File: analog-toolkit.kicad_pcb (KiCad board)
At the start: 2 copper layers, 50 x 36 mm, 54 parts, among them J1 USB_C, J2 IO, J3 UART, J4 I2C, J5 VBUS, J6 3.3V, J7 OPAMP, J8 ADC, P1 TC2030, SW1 DFU, U1 AP2204R-3.3, U2 otter_USBLC6-4, U3 STM32G431KBT6

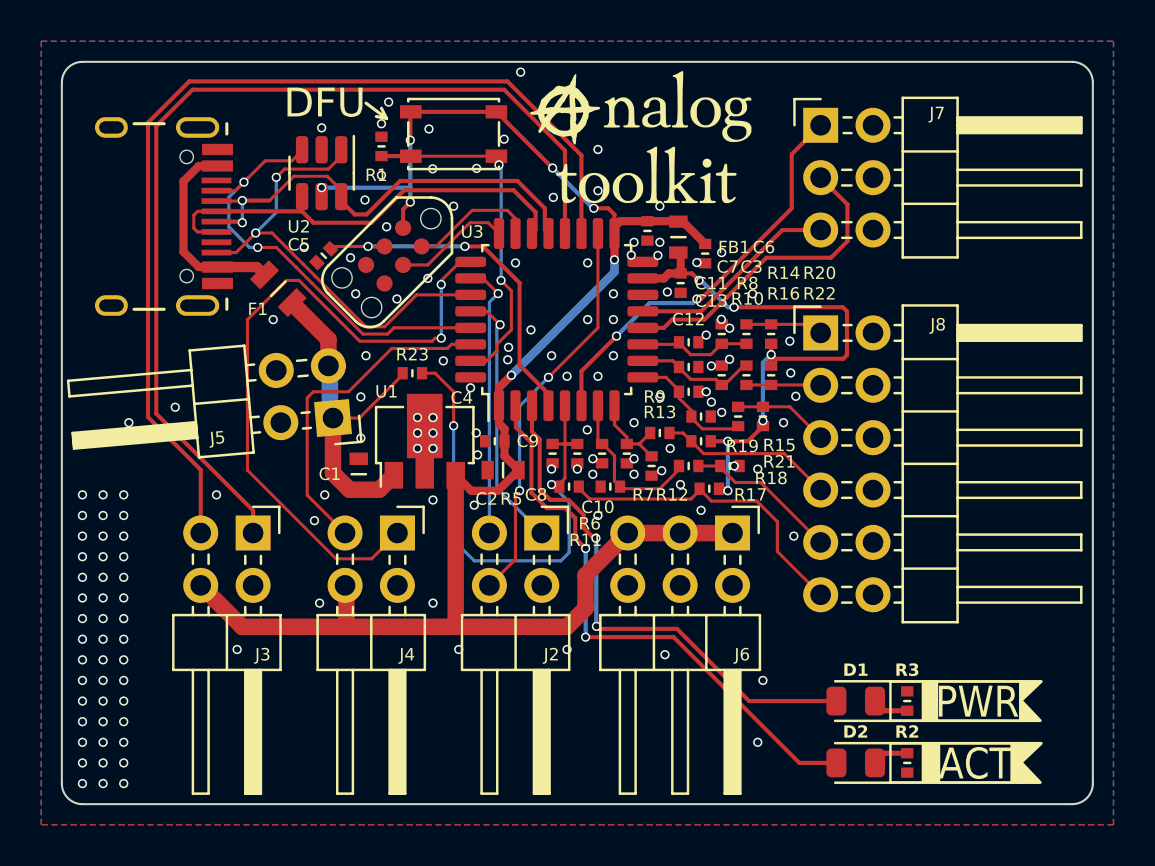
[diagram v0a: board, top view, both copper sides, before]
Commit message: added r3
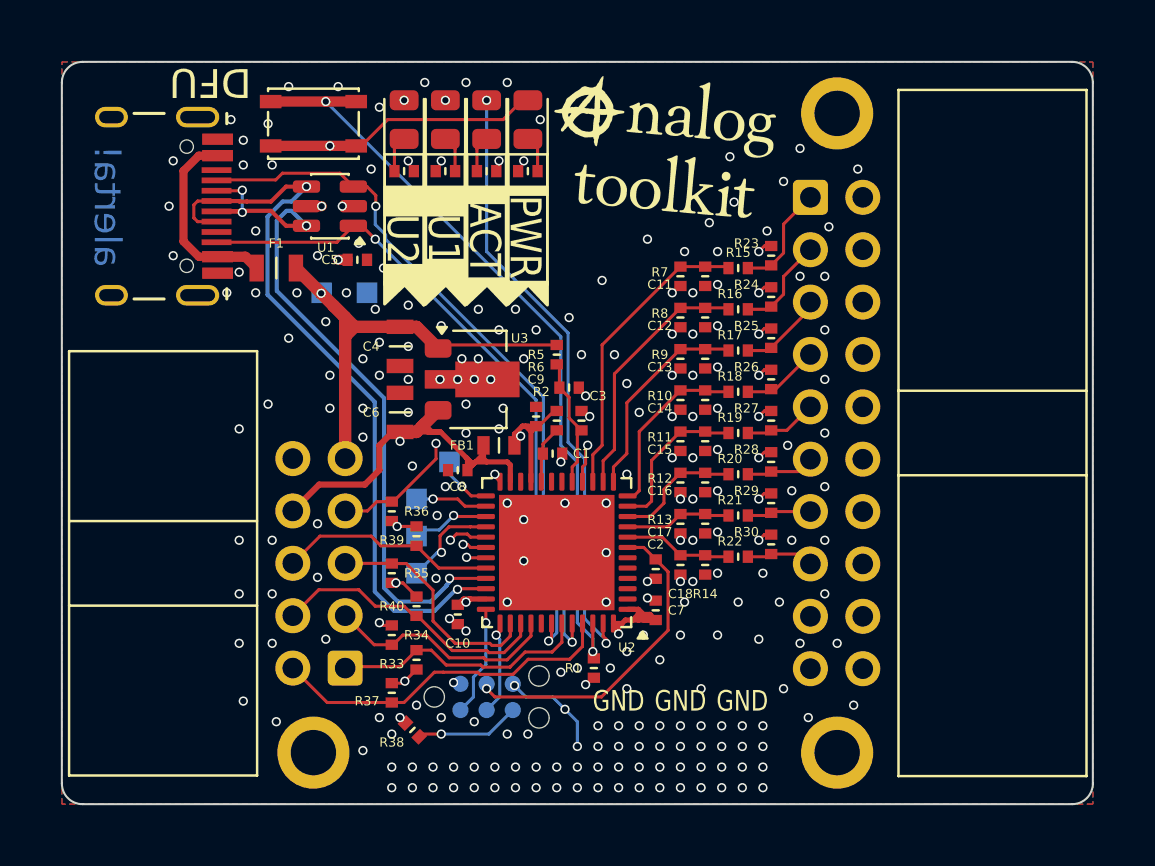
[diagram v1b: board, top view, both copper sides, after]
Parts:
- removed J4: I2C, Connector_PinHeader_2.54mm:PinHeader_2x02_P2.54mm_Horizontal
- removed J5: VBUS, Connector_PinHeader_2.54mm:PinHeader_2x02_P2.54mm_Horizontal
- removed J6: 3.3V, Connector_PinHeader_2.54mm:PinHeader_2x03_P2.54mm_Horizontal
- removed J7: OPAMP, Connector_PinHeader_2.54mm:PinHeader_2x03_P2.54mm_Horizontal
- removed J8: ADC, Connector_PinHeader_2.54mm:PinHeader_2x06_P2.54mm_Horizontal
- added C14: 10n, otter:C_0402, F.Cu at (130.0, 116.4)
- added C15: 10n, otter:C_0402, F.Cu at (130.0, 118.4)
- added C16: 10n, otter:C_0402, F.Cu at (130.0, 120.4)
- added C17: 10n, otter:C_0402, F.Cu at (130.0, 122.4)
- added C18: 10n, otter:C_0402, F.Cu at (130.0, 124.4)
- added D3: USB, LED_SMD:LED_0805_2012Metric, F.Cu at (118.6, 102.8)
- added D4: ERR, LED_SMD:LED_0805_2012Metric, F.Cu at (116.6, 102.8)
- added H1: MountingHole_Pad, MountingHole:MountingHole_2.2mm_M2_ISO7380_Pad, F.Cu at (137.6, 102.5)
- added H2: MountingHole_Pad, MountingHole:MountingHole_2.2mm_M2_ISO7380_Pad, F.Cu at (112.2, 133.5)
- added H3: MountingHole_Pad, MountingHole:MountingHole_2.2mm_M2_ISO7380_Pad, F.Cu at (137.6, 133.5)
- added R24: DNP, otter:R_0402, F.Cu at (134.4, 111.4)
- added R25: DNP, otter:R_0402, F.Cu at (134.4, 113.4)
- added R26: DNP, otter:R_0402, F.Cu at (134.4, 115.4)
- added R27: DNP, otter:R_0402, F.Cu at (134.4, 117.4)
- added R28: DNP, otter:R_0402, F.Cu at (134.4, 119.4)
- added R29: DNP, otter:R_0402, F.Cu at (134.4, 121.4)
- added R30: DNP, otter:R_0402, F.Cu at (134.4, 123.4)
- added R31: 22k, otter:R_0402, F.Cu at (118.6, 105.3)
- added R32: 22k, otter:R_0402, F.Cu at (116.6, 105.3)
- added R33: DNP, otter:R_0402, F.Cu at (117.2, 129.0)
- added R34: DNP, otter:R_0402, F.Cu at (116.0, 127.8)
- added R35: DNP, otter:R_0402, F.Cu at (116.0, 124.8)
- added R36: DNP, otter:R_0402, F.Cu at (116.0, 121.8)
- added R37: DNP, otter:R_0402, F.Cu at (116.0, 130.6)
- added R38: DNP, otter:R_0402, F.Cu at (117.0, 132.4)
- added R39: DNP, otter:R_0402, F.Cu at (117.2, 123.0)
- added R4: 22k, otter:R_0402, F.Cu at (120.6, 105.3)
- added R40: DNP, otter:R_0402, F.Cu at (117.2, 126.4)
- added TP1: TestPoint, TestPoint:TestPoint_Pad_1.0x1.0mm, B.Cu at (118.8, 119.4)
- added TP2: TestPoint, TestPoint:TestPoint_Pad_1.0x1.0mm, B.Cu at (117.2, 121.2)
- added TP3: TestPoint, TestPoint:TestPoint_Pad_1.0x1.0mm, B.Cu at (117.2, 123.0)
- added TP4: TestPoint, TestPoint:TestPoint_Pad_1.0x1.0mm, B.Cu at (117.2, 124.8)
- added TP5: TestPoint, TestPoint:TestPoint_Pad_1.0x1.0mm, B.Cu at (122.4, 124.2)
- added TP6: TestPoint, TestPoint:TestPoint_Pad_1.0x1.0mm, B.Cu at (122.4, 122.2)
- added TP7: TestPoint, TestPoint:TestPoint_Pad_1.0x1.0mm, B.Cu at (112.6, 111.2)
- added TP8: TestPoint, TestPoint:TestPoint_Pad_1.0x1.0mm, B.Cu at (114.8, 111.2)
- C1: value 4u7 -> 1u; footprint otter:C_0603 -> otter:C_0402
- C10, C8, C9: value 10n -> 1u
- C2: value 4u7 -> 100n; footprint otter:C_0603 -> otter:C_0402
- C3: value 100n -> 10n
- C4, C6: value 100n -> 4u7; footprint otter:C_0402 -> otter:C_0805
- C5, C7: value 100n -> 1u
- J2: value IO -> PA; footprint Connector_PinHeader_2.54mm:PinHeader_2x02_P2.54mm_Horizontal -> Connector_IDC:IDC-Header_2x10_P2.54mm_Horizontal
- J3: value UART -> PC/PB; footprint Connector_PinHeader_2.54mm:PinHeader_2x02_P2.54mm_Horizontal -> Connector_IDC:IDC-Header_2x05_P2.54mm_Horizontal
- P1: moved to B.Cu
- R11, R12, R13, R14: value 0 -> DNP
- R17, R18, R19, R20, R21, R22: value DNP -> 0
- R2: value 22k -> DNP
- R5: value DNP -> 22k
- R6: value DNP -> 2k2
- U1: value AP2204R-3.3 -> otter_USBLC6-4; footprint Package_TO_SOT_SMD:SOT-89-3 -> Package_TO_SOT_SMD:SOT-23-6
- U2: value otter_USBLC6-4 -> STM32G474CCUx; footprint Package_TO_SOT_SMD:SOT-23-6 -> Package_DFN_QFN:QFN-48-1EP_7x7mm_P0.5mm_EP5.6x5.6mm
- U3: value STM32G431KBT6 -> AP2204R-3.3; footprint Package_QFP:LQFP-32_7x7mm_P0.8mm -> Package_TO_SOT_SMD:SOT-89-3
- moved D2 36.0 mm to (120.6, 102.8), turned to 90 degrees
- moved D1 32.4 mm to (122.6, 102.8), turned to 90 degrees
- moved R3 31.6 mm to (122.6, 105.3), turned to 180 degrees
- moved R1 27.3 mm to (125.8, 129.4), turned to -90 degrees
- moved R2 23.8 mm to (124.0, 117.4), turned to 90 degrees
- moved P1 21.9 mm to (120.6, 130.8), turned to 0 degrees
- moved U2 21.6 mm to (124.0, 123.8), turned to 180 degrees
- moved J2 20.9 mm to (136.3, 106.6), turned to 0 degrees
- moved R23 18.3 mm to (134.4, 109.4), turned to 90 degrees
- moved C7 15.9 mm to (128.8, 126.6), turned to 90 degrees
- moved C6 14.9 mm to (116.4, 117.0), turned to 90 degrees
- moved FB1 13.3 mm to (121.2, 118.6), turned to 0 degrees
- moved U1 12.3 mm to (113.0, 107.0), turned to 180 degrees
- moved R14 11.4 mm to (131.2, 124.4)
- moved C10 11.3 mm to (119.2, 126.8)
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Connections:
- C1 pad 1: VBUS -> Net-(U2-VREF+)
- C10 pad 1: ADC1_4 -> +3V3
- C11 pad 1: ADC2_3 -> ADC2_IN4/COMP2_INP_OUT/OPAMP1_2_VINP
- C12 pad 1: ADC2_17 -> ADC2_IN3/COMP1_OUT/DAC2_OUT1/OPAMP2_VOUT
- C13 pad 1: ADC2_13 -> ADC2_IN13/COMP2_INM/DAC1_OUT2/OPAMP2_VINM
- C2 pad 1: +3V3 -> GND
- C2 pad 2: GND -> nRST
- C3 pad 1: +3V3 -> VBUS_ADC
- C4 pad 1: +3V3 -> VBUS
- C5 pad 1: GND -> +3V3
- C5 pad 2: nRST -> GND
- C7 pad 1: +3.3VA -> +3V3
- C8 pad 1: ADC1_1 -> +3V3
- C9 pad 1: ADC1_3 -> +3.3VA
- D1 pad 2: LED2 -> +3V3
- D2 pad 2: LED1 -> LED2
- J2 pad 1: TIM3_CH2 -> Net-(J2-Pin_1)
- J2 pad 2: GND -> +3.3VA
- J2 pad 3: TIM2_CH2 -> Net-(J2-Pin_3)
- J2 pad 4: PA8 -> GND
- J3 pad 1: UART_RX -> PB5
- J3 pad 2: GND -> PB7
- J3 pad 3: UART_TX -> PC11
- J3 pad 4: +3V3 -> PC10
- P1 pad 6: unconnected-(P1-SWO/TDO-Pad6) -> Net-(P1-SWO/TDO)
- R1 pad 1: Net-(U3-PB8-BOOT0) -> Net-(U2-PB8)
- R10 pad 2: ADC2_13 -> ADC2_IN17/COMP1_INM/DAC1_OUT1
- R11 pad 1: ADC1_1 -> GND
- R11 pad 2: Net-(J8-Pin_11) -> ADC1_IN4/OPAMP1_VINM_VINP/OPAMP5_VINM
- R12 pad 1: ADC1_3 -> GND
- R12 pad 2: Net-(J8-Pin_9) -> ADC1_IN3/COMP2_INM_OUT/OPAMP1_VOUT
- R13 pad 1: ADC1_4 -> GND
- R13 pad 2: Net-(J8-Pin_7) -> ADC1_IN2/ADC2_IN2/COMP1_INP/OPAMP1_2_VINP/OPAMP6_VINM
- R14 pad 1: ADC2_3 -> GND
- R14 pad 2: Net-(J8-Pin_1) -> ADC1_IN1/ADC2_IN1/COMP1_INM_OUT/COMP3_INP
- R15 pad 1: ADC2_17 -> ADC2_IN4/COMP2_INP_OUT/OPAMP1_2_VINP
- R15 pad 2: Net-(J8-Pin_5) -> Net-(J2-Pin_1)
- R16 pad 1: ADC2_13 -> ADC2_IN3/COMP1_OUT/DAC2_OUT1/OPAMP2_VOUT
- R16 pad 2: Net-(J8-Pin_3) -> Net-(J2-Pin_3)
- R17 pad 1: Net-(J8-Pin_11) -> ADC2_IN13/COMP2_INM/DAC1_OUT2/OPAMP2_VINM
- R17 pad 2: +3.3VA -> Net-(J2-Pin_5)
- R18 pad 1: Net-(J8-Pin_9) -> ADC2_IN17/COMP1_INM/DAC1_OUT1
- R18 pad 2: +3.3VA -> Net-(J2-Pin_7)
- R19 pad 1: Net-(J8-Pin_7) -> ADC1_IN4/OPAMP1_VINM_VINP/OPAMP5_VINM
- R19 pad 2: +3.3VA -> Net-(J2-Pin_9)
- R2 pad 1: Net-(D2-K) -> Net-(U2-VREF+)
- R2 pad 2: GND -> +3.3VA
- R20 pad 1: Net-(J8-Pin_1) -> ADC1_IN3/COMP2_INM_OUT/OPAMP1_VOUT
- R20 pad 2: +3.3VA -> Net-(J2-Pin_11)
- R21 pad 1: Net-(J8-Pin_5) -> ADC1_IN2/ADC2_IN2/COMP1_INP/OPAMP1_2_VINP/OPAMP6_VINM
- R21 pad 2: +3.3VA -> Net-(J2-Pin_13)
- R22 pad 1: Net-(J8-Pin_3) -> ADC1_IN1/ADC2_IN1/COMP1_INM_OUT/COMP3_INP
- R22 pad 2: +3.3VA -> Net-(J2-Pin_15)
- R23 pad 1: ADC1_1 -> Net-(J2-Pin_1)
- R23 pad 2: VBUS -> +3.3VA
- R3 pad 1: GND -> Net-(D1-K)
- R3 pad 2: Net-(D1-K) -> GND
- R5 pad 1: GND -> VBUS_ADC
- R5 pad 2: ADC1_1 -> VBUS
- R6 pad 2: ADC1_3 -> VBUS_ADC
- R7 pad 2: ADC1_4 -> ADC2_IN4/COMP2_INP_OUT/OPAMP1_2_VINP
- R8 pad 2: ADC2_3 -> ADC2_IN3/COMP1_OUT/DAC2_OUT1/OPAMP2_VOUT
- R9 pad 2: ADC2_17 -> ADC2_IN13/COMP2_INM/DAC1_OUT2/OPAMP2_VINM
- SW1 pad 1: Net-(U3-PB8-BOOT0) -> Net-(U2-PB8)
- U1 pad 1: VBUS -> CC2
- U1 pad 3: +3V3 -> CC1
- U2 pad 1: CC2 -> +3V3
- U2 pad 2: GND -> unconnected-(U2-PC13-Pad2)
- U2 pad 3: CC1 -> unconnected-(U2-PC14-Pad3)
- U2 pad 4: D+ -> unconnected-(U2-PC15-Pad4)
- U2 pad 5: +3V3 -> unconnected-(U2-PF0-Pad5)
- U2 pad 6: D- -> unconnected-(U2-PF1-Pad6)
- U3 pad 1: +3V3 -> VBUS
- U3 pad 2: LED1 -> GND
- U3 pad 3: LED2 -> +3V3
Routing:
- net VBUS: track 16.9 -> 72.9 mm, vias 0 -> 1
- net UART_TX: track 48.1 -> 0.00 mm
- net UART_RX: track 47.5 -> 0.00 mm
- net Net-(U2-PB8): track 0.00 -> 37.9 mm, vias 0 -> 2
- net I2C_SCL: track 32.9 -> 0.00 mm, vias 2 -> 0
- net PC4: track 0.00 -> 27.3 mm, vias 0 -> 3
- net ADC1_1: track 25.2 -> 0.00 mm, vias 2 -> 0
- net +3.3VA: track 28.7 -> 53.5 mm, vias 7 -> 9
- net LED4: track 0.00 -> 21.6 mm, vias 0 -> 2
- net HRTIM1_CHA2: track 0.00 -> 19.9 mm, vias 0 -> 1
- net HRTIM1_CHA1: track 0.00 -> 19.8 mm, vias 0 -> 1
- net OPAMP1: track 19.8 -> 0.00 mm, vias 2 -> 0
- net PA8: track 19.2 -> 0.00 mm, vias 2 -> 0
- net Net-(U3-PB8-BOOT0): track 17.1 -> 0.00 mm, vias 2 -> 0
- net PB7: track 0.00 -> 17.1 mm
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- added copper zone on In1.Cu, net GND
- added copper zone on In2.Cu, net GND
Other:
- copper layers 2 -> 4
- board text added: "3VA3"
- board text added: "Jana M. Hemsing 2026.03"
- board text added: "PA0"
- board text added: "PA1"
- board text added: "PA10"
- board text added: "PA15"
- board text added: "PA2"
- board text added: "PA3"
- board text added: "PA4"
- board text added: "PA5"
- board text added: "PA6"
- board text added: "PA7"
- board text added: "PA9"
- board text added: "PB12"
- board text added: "PB13"
- board text added: "PB14"
- board text added: "PB15"
- board text added: "PB5"
- board text added: "PB7"
- board text added: "PC10"
- board text added: "PC11"
- board text added: "PC4"
- board text added: "STM32G474 Analog toolkit r3"
- board text added: "U1"
- board text added: "U2"
- board text added: "alerta!"
- board text removed: "3.3V"
- board text removed: "AD14 AD13 AD11"
- board text removed: "AD23 A213 A217"
- board text removed: "ADC x6, PGA x3, IO x3, TIM x2, I2C, UART & USB-PD"
- board text removed: "OP1 OP2 OP3"
- board text removed: "RX TX"
- board text removed: "SCL SDA"
- board text removed: "STM32G4 Analog toolkit Jana Marie 2026"
- board text removed: "T3C2 T2C2"
